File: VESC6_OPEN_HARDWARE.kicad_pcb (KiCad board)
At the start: 2 copper layers, 112.6 x 46.7 mm, 125 parts, among them P1 USB_OTG, P10 PH_A, P11 SUPPLY, P12 GND, P2 TS_CAN, P3 SWD, P4 HALL/Encoder, P5 TS_CAN, P7 Custom, P8 PH_C, P9 PH_B, Q1 STL130N6F7, Q2 STL130N6F7, Q3 STL130N6F7, Q4 STL130N6F7, Q5 STL130N6F7, Q6 STL130N6F7, U1 STM32F40X_LQFP64, U10 LSM6DS3TR-C, U2 LM3671, U3 DRV8301, U4 TJA1051TK-3, U5 AD8418, U6 AD8418, U7 AD8418, X1 8m

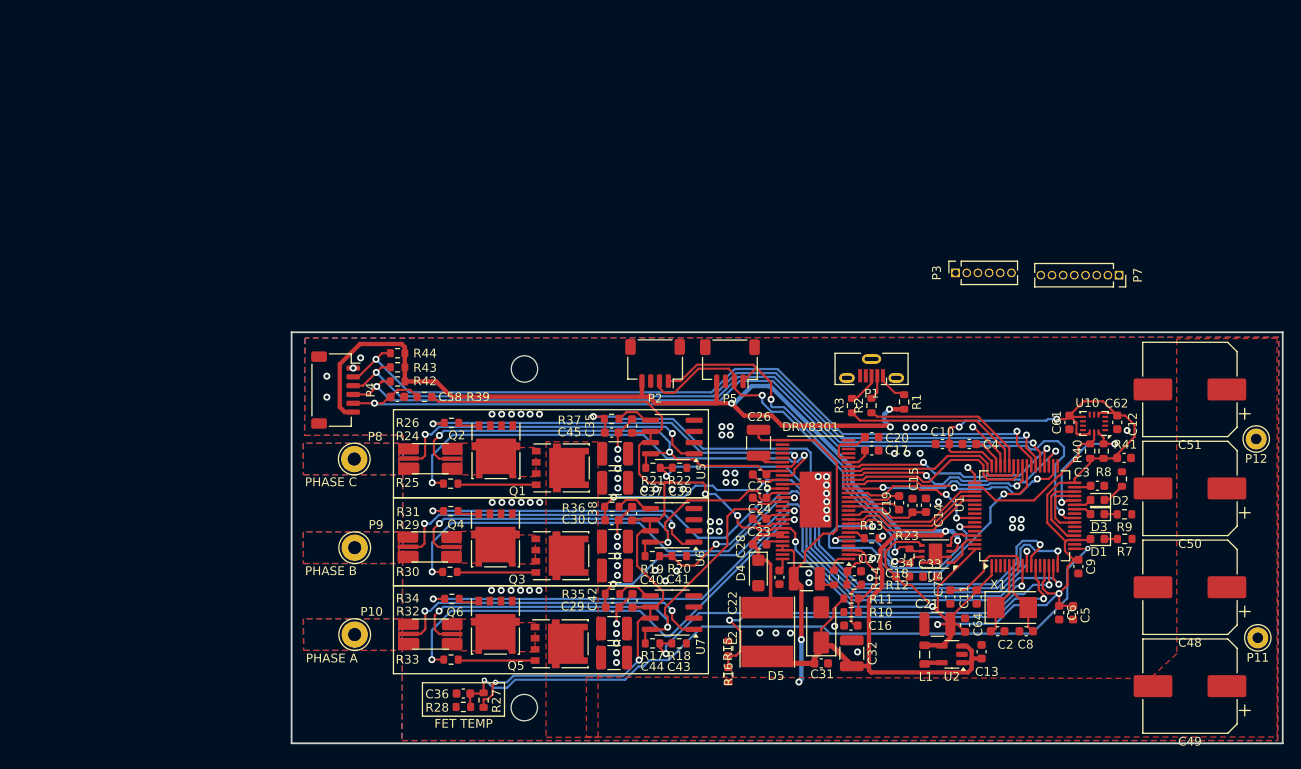
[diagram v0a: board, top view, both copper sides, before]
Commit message: Adjusted connectors and routing
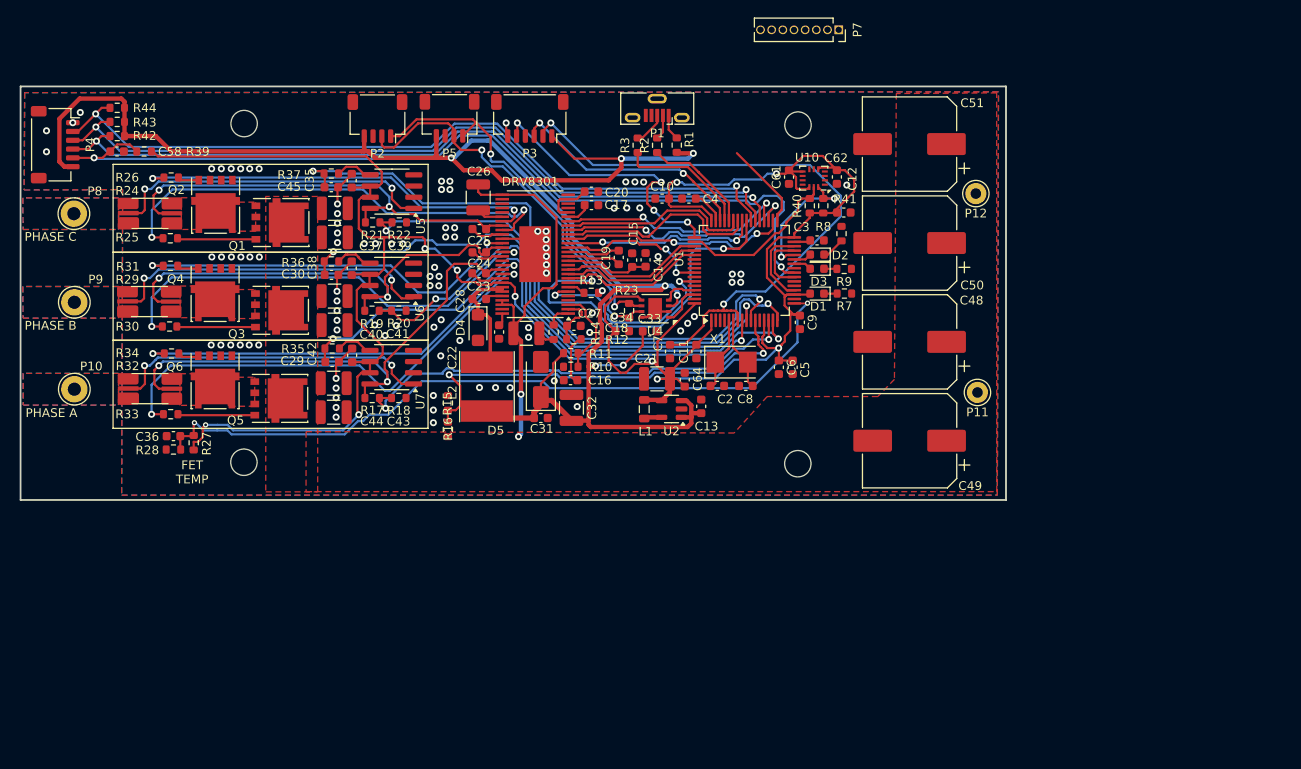
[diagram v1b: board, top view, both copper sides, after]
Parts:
- P3: footprint Connector_PinSocket_1.27mm:PinSocket_1x06_P1.27mm_Vertical -> Connector_JST:JST_SH_SM06B-SRSS-TB_1x06-1MP_P1.00mm_Horizontal
- moved P3 51.5 mm to (57.9, 3.63), turned to 180 degrees
- moved C36 44.1 mm to (17.4, 39.7)
- moved R27 44.1 mm to (19.7, 40.5)
- moved R28 44.1 mm to (17.4, 41.3)
- moved C12 42.3 mm to (93.6, 14.3)
- moved C14 42.3 mm to (71.0, 19.7)
- moved C16 42.3 mm to (62.5, 33.4)
- moved C18 42.3 mm to (62.9, 27.2)
- moved C21 42.3 mm to (72.3, 33.2)
- moved C24 42.3 mm to (52.1, 18.9)
- moved C25 42.3 mm to (52.1, 16.2)
- moved C26 42.3 mm to (52.0, 12.6)
- moved C29 42.3 mm to (35.4, 31.3)
- moved C31 42.3 mm to (59.1, 37.7)
- moved C4 42.3 mm to (76.0, 12.8)
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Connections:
- P3 pad 1: VCC -> +5V
- P3 pad 2: /stm32f40x/SWCLK -> /stm32f40x/NRST
- P3 pad 3: GND -> /stm32f40x/SWDIO
- P3 pad 4: /stm32f40x/SWDIO -> GND
- P3 pad 5: /stm32f40x/NRST -> /stm32f40x/SWCLK
- P3 pad 6: unconnected-(P3-Pin_6-Pad6) -> VCC
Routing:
- net /stm32f40x/NRST: track 11.0 -> 69.8 mm, vias 0 -> 2
- net /stm32f40x/SWCLK: track 2.06 -> 31.8 mm, vias 1 -> 4
- net +5V: track 182.0 -> 209.2 mm, vias 5 -> 7
- net /stm32f40x/SWDIO: track 5.78 -> 27.7 mm, vias 1 -> 2
- net /stm32f40x/PB12: track 0.00 -> 9.98 mm
- net VCC: track 270.5 -> 277.6 mm, vias 10 -> 11
- net /stm32f40x/USB_DM: track 19.4 -> 12.6 mm
- net /stm32f40x/USB_DP: track 21.0 -> 15.0 mm
- net /DRV8301/CS: track 40.9 -> 42.7 mm
- net /power/TEMP: track 84.2 -> 85.1 mm
- net Net-(P1-VBUS): track 3.66 -> 2.93 mm
- net /DRV8301/SENS_A: track 52.3 -> 52.9 mm
- net GND: vias 85 -> 96
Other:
- board size 112.6 x 46.7 mm -> 112 x 47 mm
- board text added: "ADC port EN_BUCK switch"
- board text removed: "ADC port Aditional CAN port for BMS"
